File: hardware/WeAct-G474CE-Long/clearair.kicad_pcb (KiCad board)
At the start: 2 copper layers, 116.6 x 58.4 mm, 35 parts, among them J3 SPS30 wire header (1 VDD, 2 S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, J4 BME680 wire header (1 VCC, 2 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, J5 MQ131 wire header (1 VCC, 2 G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, J6 MiCS-4514 wire header (1 VCC,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, J7 RTC PCF8563, M2 80mm fan front, M3 80mm fan rear, Q1 2N7000, Q2 2N7000, Q3 2N2222A, SW1 RESET, SW2 COLD_BOOT, U5 RobotDyn AC dimmer

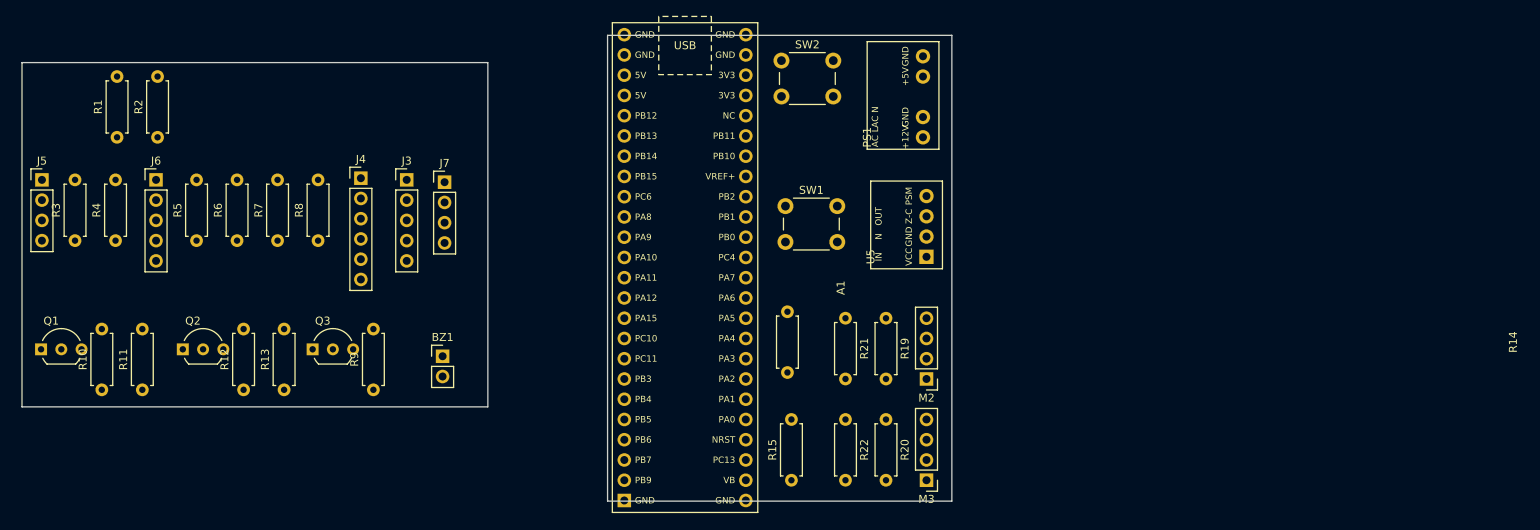
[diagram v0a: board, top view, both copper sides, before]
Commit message: fix layout and script generators
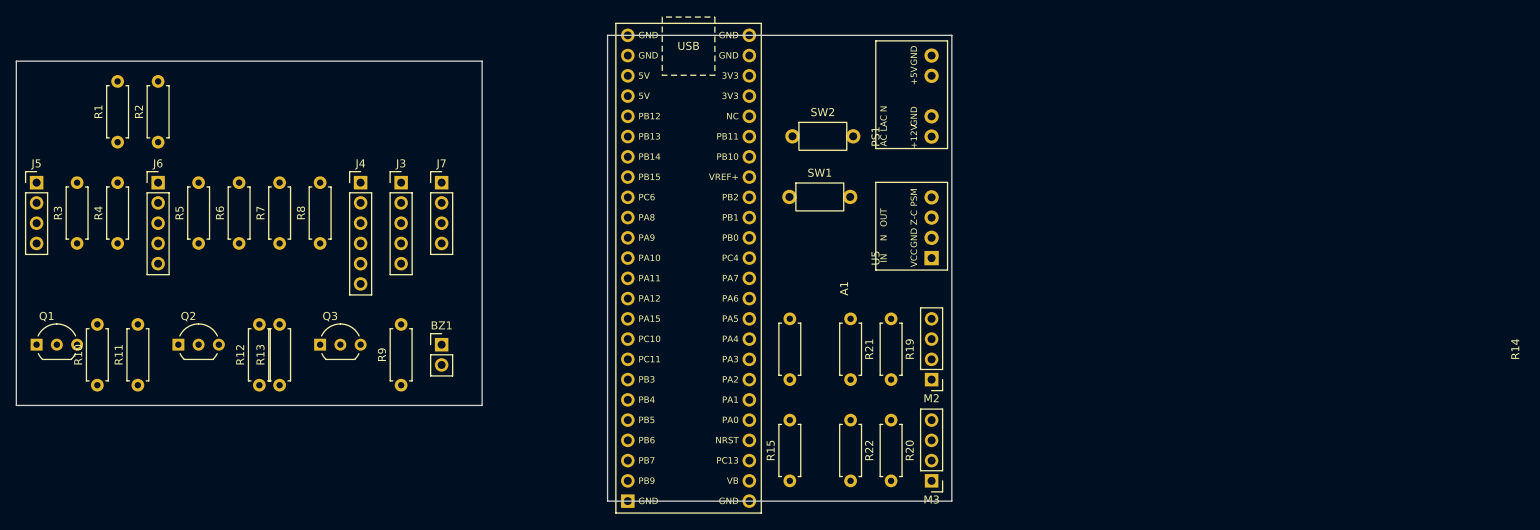
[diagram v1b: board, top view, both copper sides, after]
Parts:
- SW1: value RESET -> RESET red; footprint Button_Switch_THT:SW_PUSH_6mm -> SW_Tactile_3x6_2pin
- SW2: value COLD_BOOT -> COLD_BOOT white; footprint Button_Switch_THT:SW_PUSH_6mm -> SW_Tactile_3x6_2pin
- moved SW2 9.60 mm to (201.6, 71.2)
- moved R9 3.53 mm to (152.6, 102.5)
- moved R12 2.06 mm to (134.8, 102.5)
- moved BZ1 1.45 mm to (157.6, 97.4)
- moved SW1 1.25 mm to (201.2, 78.8)
- moved Q3 1.10 mm to (142.4, 97.4)
- moved PS1 1.08 mm to (219.1, 71.3)
- moved R14 0.94 mm to (201.3, 101.8)
- moved R10 0.81 mm to (114.5, 102.5)
- moved R11 0.81 mm to (119.5, 102.5)
- moved R13 0.81 mm to (137.3, 102.5)
- moved Q1 0.81 mm to (106.8, 97.4)
- moved Q2 0.81 mm to (124.6, 97.4)
- moved J3 0.78 mm to (152.6, 77.1)
- moved J5 0.76 mm to (106.8, 77.1)
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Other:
- board size 116.6 x 58.4 mm -> 117.3 x 58.4 mm
